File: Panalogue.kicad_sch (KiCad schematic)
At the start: 28 parts, among them J1 Y/C video, J2 CVBS video, J3 Conn_A23_Edge_Pads, SW1 NTSC/PAL, SW2 NTSC/PAL, U1 CXA2075M

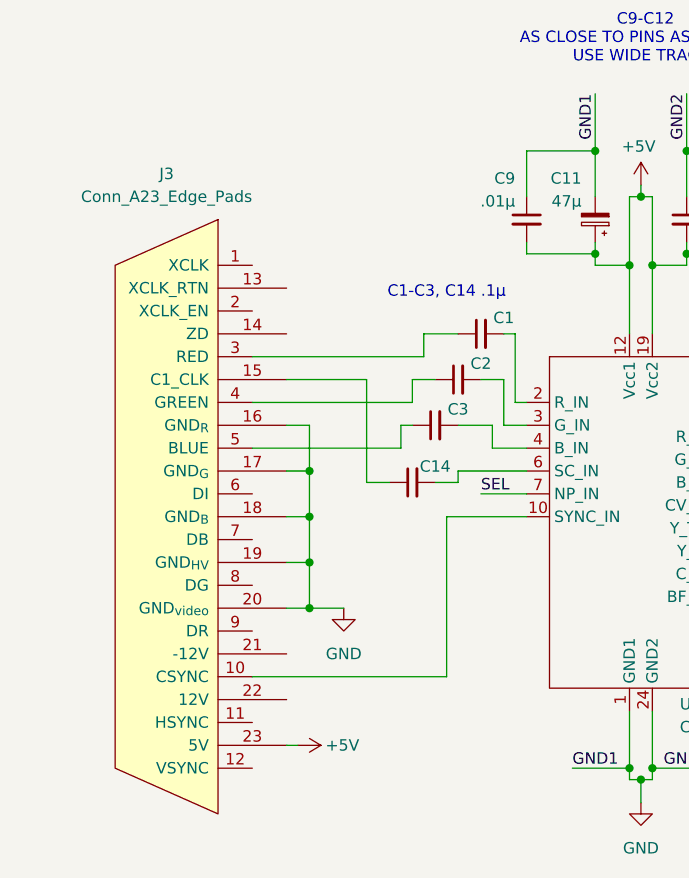
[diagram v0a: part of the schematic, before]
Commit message: first complete schematic
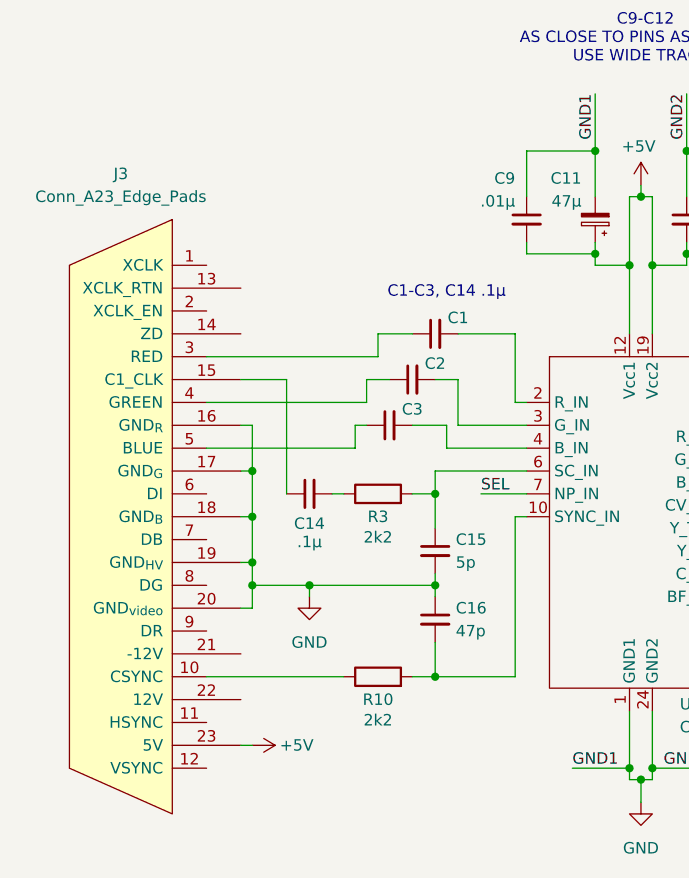
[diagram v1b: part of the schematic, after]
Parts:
- added C15: 5p, Capacitor_THT:C_Disc_D3.0mm_W1.6mm_P2.50mm, symbol Device:C_Small
- added C16: 47p, Capacitor_THT:C_Disc_D3.0mm_W1.6mm_P2.50mm, symbol Device:C_Small
- added R10, R3: 2k2, Resistor_THT:R_Axial_DIN0204_L3.6mm_D1.6mm_P7.62mm_Horizontal, symbol Device:R
- C1, C10, C14, C2, C3, C9: footprint (none) -> Capacitor_THT:C_Disc_D3.0mm_W1.6mm_P2.50mm
- J1: footprint (none) -> Connector_Mini-DIN:Mini-DIN_4_KMDGX4SBS
- J2: footprint (none) -> Connector_Audio_Custom:Jack_Phono_CUI_RCJ044
- J3: footprint (none) -> Amiga:D_23_Socket_EdgeMount
- R1, R2, R4, R5, R6, R7, R8, R9: footprint (none) -> Resistor_THT:R_Axial_DIN0204_L3.6mm_D1.6mm_P7.62mm_Horizontal
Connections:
- net GND: now also C15.2, C16.1
- net at C14.2: now also R3.1; no longer U1.6 (SC_IN)
- net at J3.10 (CSYNC): now also R10.1; no longer U1.10 (SYNC_IN)
- new net: C16.2, R10.2, U1.10 (SYNC_IN)
- new net: C15.1, R3.2, U1.6 (SC_IN)
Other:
- moved on the sheet: C1, C14, C2, C3, J3
